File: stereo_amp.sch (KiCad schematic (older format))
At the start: 10 parts, among them J101 HEADER1X2, J102 HEADER1X2, J103 HEADER1X2, J104 HEADER1X2, J105 HEADER1X5, J106 VCCL, J107 VCCR, J108 HEADER1X5, J109 HEADER1X2, J110 HEADER1X2

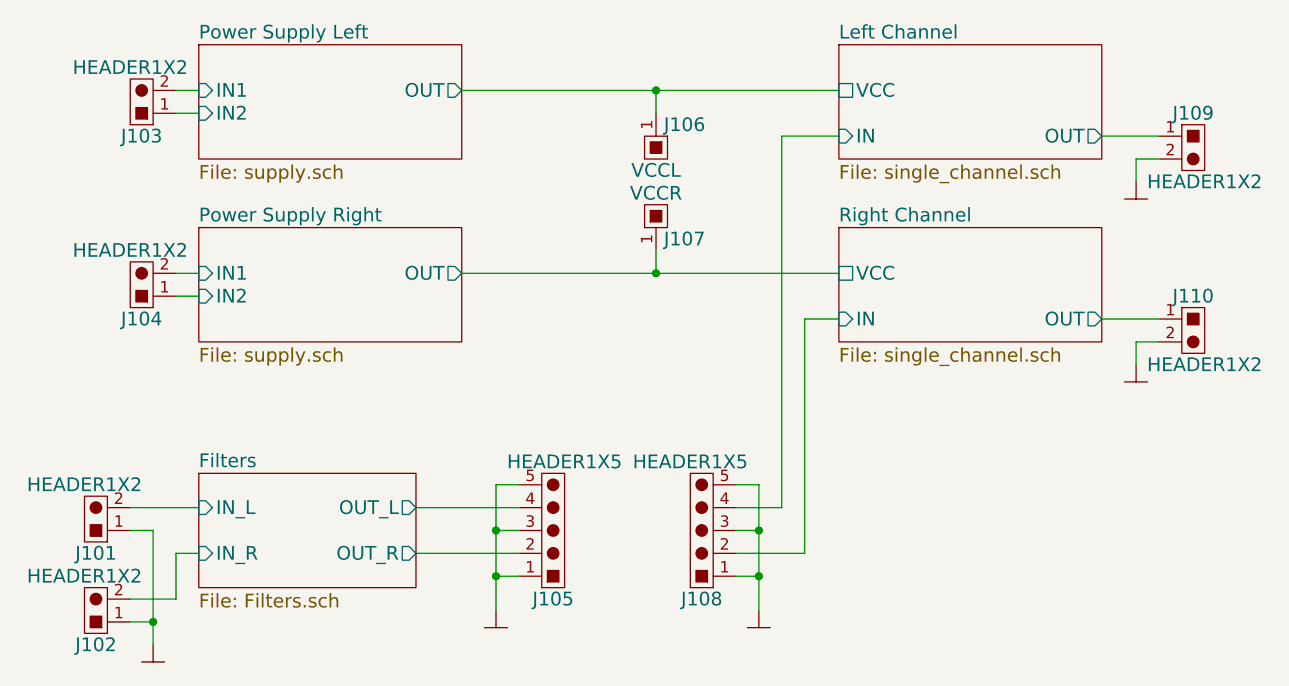
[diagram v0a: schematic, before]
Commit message: Finished placement and routing.
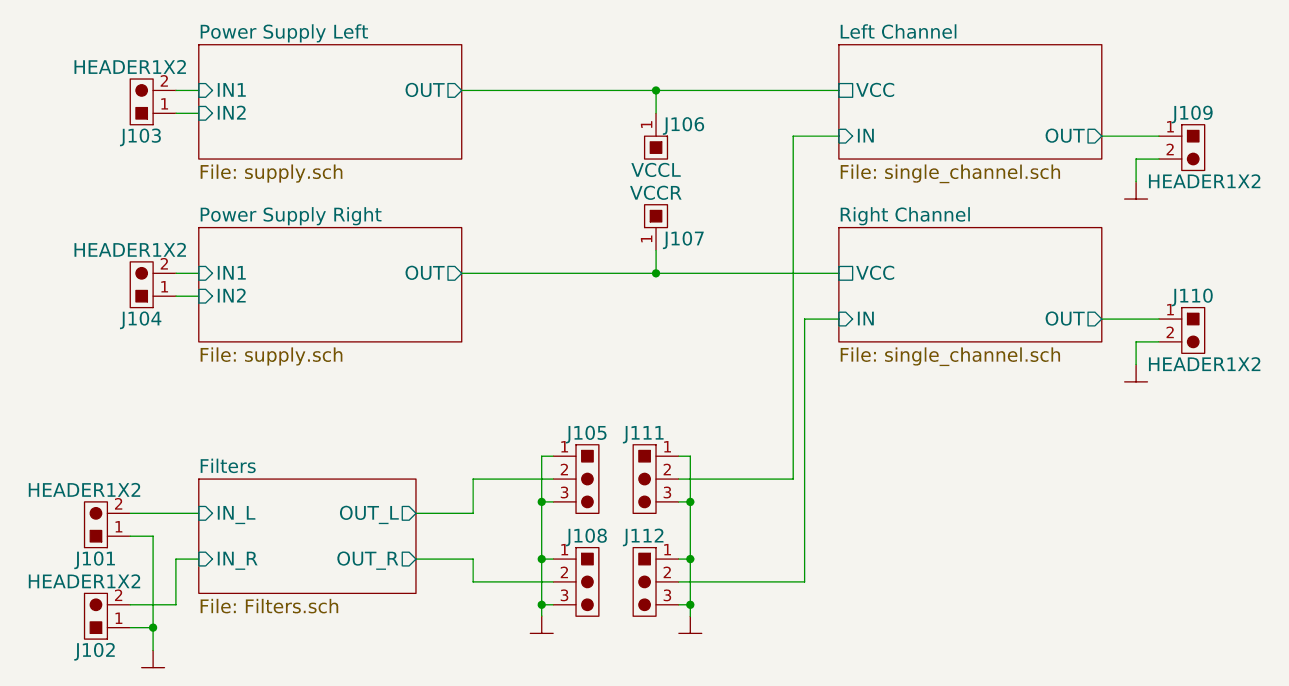
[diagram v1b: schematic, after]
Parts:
- removed J105, J108: HEADER1X5, Pinhead:HEADER1x5V, symbol HEADER1X5
- added J105, J108, J111, J112: HEADER1X3, symbol HEADER1X3
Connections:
- net Filters/OUT_L: now also J105.2
- net Filters/OUT_R: now also J108.2
- net GND: now also J105.1, J105.3, J108.1, J108.3, J111.1, J111.3, J112.1, J112.3
- net Left Channel/IN: now also J111.2
- net Right Channel/IN: now also J112.2
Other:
- moved on the sheet: J101, J102
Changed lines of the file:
@@
 $EndComp
 $Comp
-L GND #PWR01
+L GND #PWR104
 U 1 1 543EAEE5
 P 7800 4100
-F 0 "#PWR01" H 7800 4060 30  0001 C CNN
+F 0 "#PWR104" H 7800 4060 30  0001 C CNN
 F 1 "GND" H 7800 3985 30  0001 C CNN
 F 2 "" H 7800 4100 60  0000 C CNN
@@
 	7900 4700 7650 4700
 $Comp
-L GND #PWR02
+L GND #PWR105
 U 1 1 543EAF54
 P 7800 4900
-F 0 "#PWR02" H 7800 4860 30  0001 C CNN
+F 0 "#PWR105" H 7800 4860 30  0001 C CNN
 F 1 "GND" H 7800 4785 30  0001 C CNN
 F 2 "" H 7800 4900 60  0000 C CNN
@@
 Wire Wire Line
 	7800 4800 7900 4800
-$Comp
-L HEADER1X5 J108
-U 1 1 543EB287
-P 5900 5625
-F 0 "J108" H 5900 5925 60  0000 C CNN
-F 1 "HEADER1X5" H 5950 5325 60  0000 C CNN
-F 2 "Pinhead:HEADER1x5V" H 5900 5625 60  0001 C CNN
-F 3 "" H 5900 5625 60  0000 C CNN
-	1    5900 5625
-	-1   0    0    1
-$EndComp
 $Comp
 L HEADER1X2 J103
@@
 	-1   0    0    1
 $EndComp
-$Comp
-L GND #PWR03
-U 1 1 543EB64E
-P 6150 5975
-F 0 "#PWR03" H 6150 5935 30  0001 C CNN
-F 1 "GND" H 6150 5860 30  0001 C CNN
-F 2 "" H 6150 5975 60  0000 C CNN
-F 3 "" H 6150 5975 60  0000 C CNN
-	1    6150 5975
-	1    0    0    -1
-$EndComp
-Wire Wire Line
-	6050 5525 6250 5525
-Wire Wire Line
-	6050 5725 6350 5725
-Wire Wire Line
-	6050 5425 6150 5425
-Wire Wire Line
-	6150 5425 6150 5975
-Wire Wire Line
-	6050 5825 6150 5825
-Connection ~ 6150 5825
-Wire Wire Line
-	6050 5625 6150 5625
-Connection ~ 6150 5625
-$Comp
-L HEADER1X5 J105
-U 1 1 543D88B1
-P 5250 5625
-F 0 "J105" H 5250 5925 60  0000 C CNN
-F 1 "HEADER1X5" H 5300 5325 60  0000 C CNN
-F 2 "Pinhead:HEADER1x5V" H 5250 5625 60  0001 C CNN
-F 3 "" H 5250 5625 60  0000 C CNN
-	1    5250 5625
-	1    0    0    1
-$EndComp
-$Comp
-L GND #PWR04
-U 1 1 543D88E4
-P 5000 5975
-F 0 "#PWR04" H 5000 5935 30  0001 C CNN
-F 1 "GND" H 5000 5860 30  0001 C CNN
-F 2 "" H 5000 5975 60  0000 C CNN
-F 3 "" H 5000 5975 60  0000 C CNN
-	1    5000 5975
-	1    0    0    -1
-$EndComp
-Wire Wire Line
-	5000 5425 5000 5975
-Wire Wire Line
-	5000 5425 5100 5425
-Wire Wire Line
-	5100 5625 5000 5625
-Connection ~ 5000 5625
-Wire Wire Line
-	5100 5825 5000 5825
-Connection ~ 5000 5825
 $Sheet
-S 3700 5375 950  500
+S 3700 5400 950  500
 U 543D89A0
 F0 "Filters" 60
 F1 "Filters.sch" 60
-F2 "IN_L" I L 3700 5525 60
-F3 "IN_R" I L 3700 5725 60
-F4 "OUT_L" O R 4650 5525 60
-F5 "OUT_R" O R 4650 5725 60
+F2 "IN_L" I L 3700 5550 60
+F3 "IN_R" I L 3700 5750 60
+F4 "OUT_L" O R 4650 5550 60
+F5 "OUT_R" O R 4650 5750 60
 $EndSheet
-Wire Wire Line
-	4650 5725 5100 5725
-Wire Wire Line
-	4650 5525 5100 5525
 $Comp
 L HEADER1X2 J101
 U 1 1 543D94D6
-P 3250 5575
-F 0 "J101" H 3250 5725 60  0000 C CNN
-F 1 "HEADER1X2" H 3300 5425 60  0000 C CNN
-F 2 "Pinhead:HEADER1x2V" H 3250 5575 60  0001 C CNN
-F 3 "" H 3250 5575 60  0000 C CNN
-	1    3250 5575
+P 3250 5600
+F 0 "J101" H 3250 5750 60  0000 C CNN
+F 1 "HEADER1X2" H 3300 5450 60  0000 C CNN
+F 2 "Pinhead:HEADER1x2V" H 3250 5600 60  0001 C CNN
+F 3 "" H 3250 5600 60  0000 C CNN
+	1    3250 5600
 	-1   0    0    1
 $EndComp
@@
 L HEADER1X2 J102
 U 1 1 543D9570
-P 3250 5975
-F 0 "J102" H 3250 6125 60  0000 C CNN
-F 1 "HEADER1X2" H 3300 5825 60  0000 C CNN
-F 2 "Pinhead:HEADER1x2V" H 3250 5975 60  0001 C CNN
-F 3 "" H 3250 5975 60  0000 C CNN
-	1    3250 5975
-	-1   0    0    1
-$EndComp
-Wire Wire Line
-	3400 5525 3700 5525
-Wire Wire Line
-	3400 5925 3600 5925
-Wire Wire Line
-	3600 5925 3600 5725
-Wire Wire Line
-	3600 5725 3700 5725
-$Comp
-L GND #PWR05
+P 3250 6000
+F 0 "J102" H 3250 6150 60  0000 C CNN
+F 1 "HEADER1X2" H 3300 5850 60  0000 C CNN
+F 2 "Pinhead:HEADER1x2V" H 3250 6000 60  0001 C CNN
+F 3 "" H 3250 6000 60  0000 C CNN
+	1    3250 6000
+	-1   0    0    1
+$EndComp
+Wire Wire Line
+	3400 5550 3700 5550
+Wire Wire Line
+	3400 5950 3600 5950
+Wire Wire Line
+	3600 5950 3600 5750
+Wire Wire Line
+	3600 5750 3700 5750
+$Comp
+L GND #PWR101
 U 1 1 543D9631
-P 3500 6125
-F 0 "#PWR05" H 3500 6085 30  0001 C CNN
-F 1 "GND" H 3500 6010 30  0001 C CNN
-F 2 "" H 3500 6125 60  0000 C CNN
-F 3 "" H 3500 6125 60  0000 C CNN
-	1    3500 6125
-	1    0    0    -1
-$EndComp
-Wire Wire Line
-	3500 5625 3500 6125
-Wire Wire Line
-	3500 6025 3400 6025
-Wire Wire Line
-	3500 5625 3400 5625
-Connection ~ 3500 6025
+P 3500 6150
+F 0 "#PWR101" H 3500 6110 30  0001 C CNN
+F 1 "GND" H 3500 6035 30  0001 C CNN
+F 2 "" H 3500 6150 60  0000 C CNN
+F 3 "" H 3500 6150 60  0000 C CNN
+	1    3500 6150
+	1    0    0    -1
+$EndComp
+Wire Wire Line
+	3500 5650 3500 6150
+Wire Wire Line
+	3500 6050 3400 6050
+Wire Wire Line
+	3500 5650 3400 5650
+Connection ~ 3500 6050
 $Sheet
 S 3700 3500 1150 500
@@
 $EndSheet
 Wire Wire Line
-	6250 5525 6250 3900
-Wire Wire Line
-	6250 3900 6500 3900
-Wire Wire Line
-	6350 5725 6350 4700
-Wire Wire Line
-	6350 4700 6500 4700
-Wire Wire Line
 	4850 3700 6500 3700
 Wire Wire Line
@@
 	5700 4400 5700 4500
 Connection ~ 5700 4500
+$Comp
+L HEADER1X3 J105
+U 1 1 544CC4F2
+P 5400 5400
+F 0 "J105" H 5400 5600 60  0000 C CNN
+F 1 "HEADER1X3" H 5450 5200 60  0001 C CNN
+F 2 "" H 5400 5400 60  0000 C CNN
+F 3 "" H 5400 5400 60  0000 C CNN
+	1    5400 5400
+	1    0    0    -1
+$EndComp
+$Comp
+L HEADER1X3 J108
+U 1 1 544CCB12
+P 5400 5850
+F 0 "J108" H 5400 6050 60  0000 C CNN
+F 1 "HEADER1X3" H 5450 5650 60  0001 C CNN
+F 2 "" H 5400 5850 60  0000 C CNN
+F 3 "" H 5400 5850 60  0000 C CNN
+	1    5400 5850
+	1    0    0    -1
+$EndComp
+$Comp
+L HEADER1X3 J111
+U 1 1 544CCB42
+P 5650 5400
+F 0 "J111" H 5650 5600 60  0000 C CNN
+F 1 "HEADER1X3" H 5700 5200 60  0001 C CNN
+F 2 "" H 5650 5400 60  0000 C CNN
+F 3 "" H 5650 5400 60  0000 C CNN
+	1    5650 5400
+	-1   0    0    -1
+$EndComp
+$Comp
+L HEADER1X3 J112
+U 1 1 544CCB7D
+P 5650 5850
+F 0 "J112" H 5650 6050 60  0000 C CNN
+F 1 "HEADER1X3" H 5700 5650 60  0001 C CNN
+F 2 "" H 5650 5850 60  0000 C CNN
+F 3 "" H 5650 5850 60  0000 C CNN
+	1    5650 5850
+	-1   0    0    -1
+$EndComp
+Wire Wire Line
+	4650 5750 4900 5750
+Wire Wire Line
+	4900 5750 4900 5850
+Wire Wire Line
+	4900 5850 5250 5850
+Wire Wire Line
+	4650 5550 4900 5550
+Wire Wire Line
+	4900 5550 4900 5400
+Wire Wire Line
+	4900 5400 5250 5400
+Wire Wire Line
+	6500 3900 6300 3900
+Wire Wire Line
+	6300 3900 6300 5400
+Wire Wire Line
+	6300 5400 5800 5400
+Wire Wire Line
+	6500 4700 6350 4700
+Wire Wire Line
+	6350 4700 6350 5850
+Wire Wire Line
+	6350 5850 5800 5850
+$Comp
+L GND #PWR103
+U 1 1 544D174C
+P 5850 6000
+F 0 "#PWR103" H 5850 5960 30  0001 C CNN
+F 1 "GND" H 5850 5885 30  0001 C CNN
+F 2 "" H 5850 6000 60  0000 C CNN
+F 3 "" H 5850 6000 60  0000 C CNN
+	1    5850 6000
+	1    0    0    -1
+$EndComp
+$Comp
+L GND #PWR102
+U 1 1 544D1763
+P 5200 6000
+F 0 "#PWR102" H 5200 5960 30  0001 C CNN
+F 1 "GND" H 5200 5885 30  0001 C CNN
+F 2 "" H 5200 6000 60  0000 C CNN
+F 3 "" H 5200 6000 60  0000 C CNN
+	1    5200 6000
+	1    0    0    -1
+$EndComp
+Wire Wire Line
+	5200 6000 5200 5300
+Wire Wire Line
+	5200 5300 5250 5300
+Wire Wire Line
+	5250 5500 5200 5500
+Connection ~ 5200 5500
+Wire Wire Line
+	5250 5750 5200 5750
+Connection ~ 5200 5750
+Wire Wire Line
+	5250 5950 5200 5950
+Connection ~ 5200 5950
+Wire Wire Line
+	5800 5950 5850 5950
+Wire Wire Line
+	5850 5300 5850 6000
+Wire Wire Line
+	5850 5750 5800 5750
+Connection ~ 5850 5950
+Wire Wire Line
+	5850 5300 5800 5300
+Connection ~ 5850 5750
+Wire Wire Line
+	5850 5500 5800 5500
+Connection ~ 5850 5500
 $EndSCHEMATC

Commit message: Fixed transistors with swapped E-C
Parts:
- J105, J108, J111, J112: footprint (none) -> Pinhead:HEADER1x3V
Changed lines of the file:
@@
 $EndComp
 $Comp
-L GND #PWR104
+L GND #PWR01
 U 1 1 543EAEE5
 P 7800 4100
-F 0 "#PWR104" H 7800 4060 30  0001 C CNN
+F 0 "#PWR01" H 7800 4060 30  0001 C CNN
 F 1 "GND" H 7800 3985 30  0001 C CNN
 F 2 "" H 7800 4100 60  0000 C CNN
@@
 	7900 4700 7650 4700
 $Comp
-L GND #PWR105
+L GND #PWR02
 U 1 1 543EAF54
 P 7800 4900
-F 0 "#PWR105" H 7800 4860 30  0001 C CNN
+F 0 "#PWR02" H 7800 4860 30  0001 C CNN
 F 1 "GND" H 7800 4785 30  0001 C CNN
 F 2 "" H 7800 4900 60  0000 C CNN
@@
 	3600 5750 3700 5750
 $Comp
-L GND #PWR101
+L GND #PWR03
 U 1 1 543D9631
 P 3500 6150
-F 0 "#PWR101" H 3500 6110 30  0001 C CNN
+F 0 "#PWR03" H 3500 6110 30  0001 C CNN
 F 1 "GND" H 3500 6035 30  0001 C CNN
 F 2 "" H 3500 6150 60  0000 C CNN
@@
 F 0 "J105" H 5400 5600 60  0000 C CNN
 F 1 "HEADER1X3" H 5450 5200 60  0001 C CNN
-F 2 "" H 5400 5400 60  0000 C CNN
+F 2 "Pinhead:HEADER1x3V" H 5400 5400 60  0001 C CNN
 F 3 "" H 5400 5400 60  0000 C CNN
 	1    5400 5400
@@
 F 0 "J108" H 5400 6050 60  0000 C CNN
 F 1 "HEADER1X3" H 5450 5650 60  0001 C CNN
-F 2 "" H 5400 5850 60  0000 C CNN
+F 2 "Pinhead:HEADER1x3V" H 5400 5850 60  0001 C CNN
 F 3 "" H 5400 5850 60  0000 C CNN
 	1    5400 5850
@@
 F 0 "J111" H 5650 5600 60  0000 C CNN
 F 1 "HEADER1X3" H 5700 5200 60  0001 C CNN
-F 2 "" H 5650 5400 60  0000 C CNN
+F 2 "Pinhead:HEADER1x3V" H 5650 5400 60  0001 C CNN
 F 3 "" H 5650 5400 60  0000 C CNN
 	1    5650 5400
@@
 F 0 "J112" H 5650 6050 60  0000 C CNN
 F 1 "HEADER1X3" H 5700 5650 60  0001 C CNN
-F 2 "" H 5650 5850 60  0000 C CNN
+F 2 "Pinhead:HEADER1x3V" H 5650 5850 60  0001 C CNN
 F 3 "" H 5650 5850 60  0000 C CNN
 	1    5650 5850
@@
 	6350 5850 5800 5850
 $Comp
-L GND #PWR103
+L GND #PWR04
 U 1 1 544D174C
 P 5850 6000
-F 0 "#PWR103" H 5850 5960 30  0001 C CNN
+F 0 "#PWR04" H 5850 5960 30  0001 C CNN
 F 1 "GND" H 5850 5885 30  0001 C CNN
 F 2 "" H 5850 6000 60  0000 C CNN
@@
 $EndComp
 $Comp
-L GND #PWR102
+L GND #PWR05
 U 1 1 544D1763
 P 5200 6000
-F 0 "#PWR102" H 5200 5960 30  0001 C CNN
+F 0 "#PWR05" H 5200 5960 30  0001 C CNN
 F 1 "GND" H 5200 5885 30  0001 C CNN
 F 2 "" H 5200 6000 60  0000 C CNN
